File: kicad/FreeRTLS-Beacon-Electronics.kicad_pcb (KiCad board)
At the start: 2 copper layers, 27.1 x 52.5 mm, 37 parts, among them J1 USB_B_Micro, J2 STM Prog, U1 STM32F072CBTx, U2 AZ1117IH-3.3TRG1, U3 DWM1001

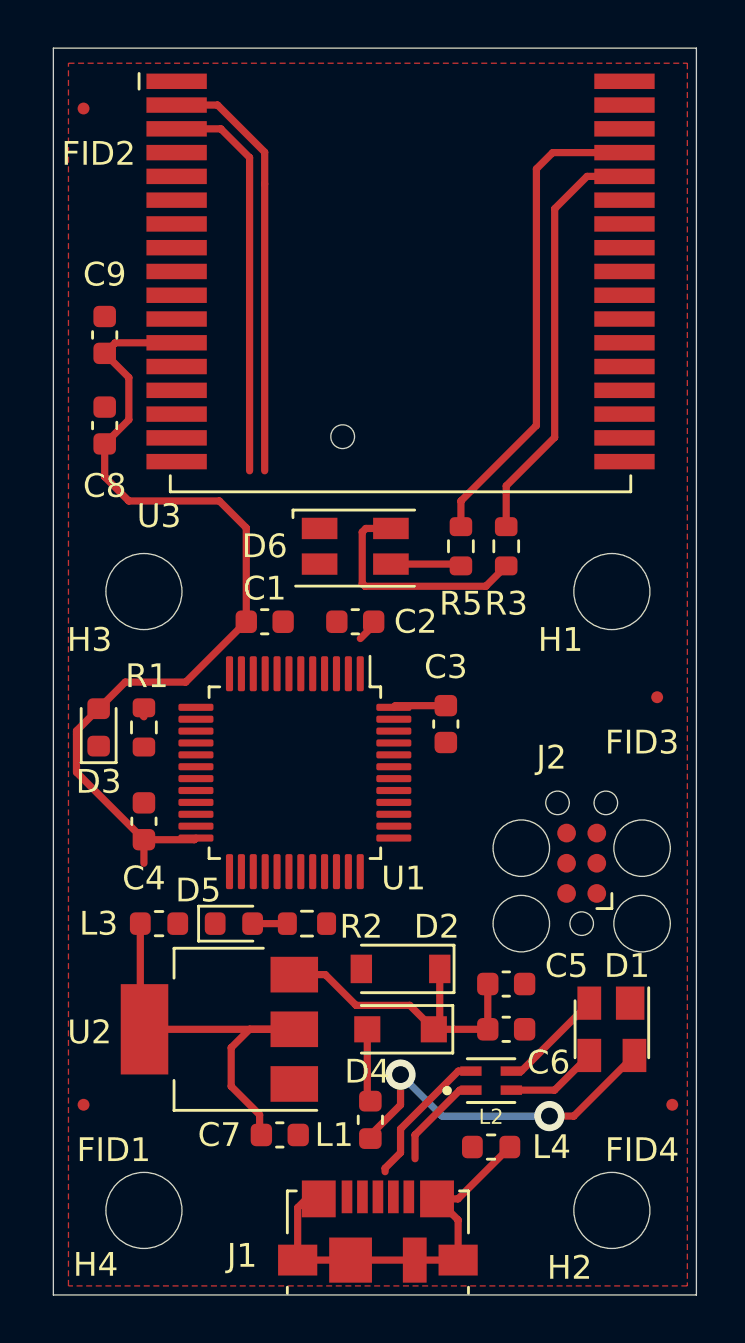
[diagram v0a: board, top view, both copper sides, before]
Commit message: Finish routing
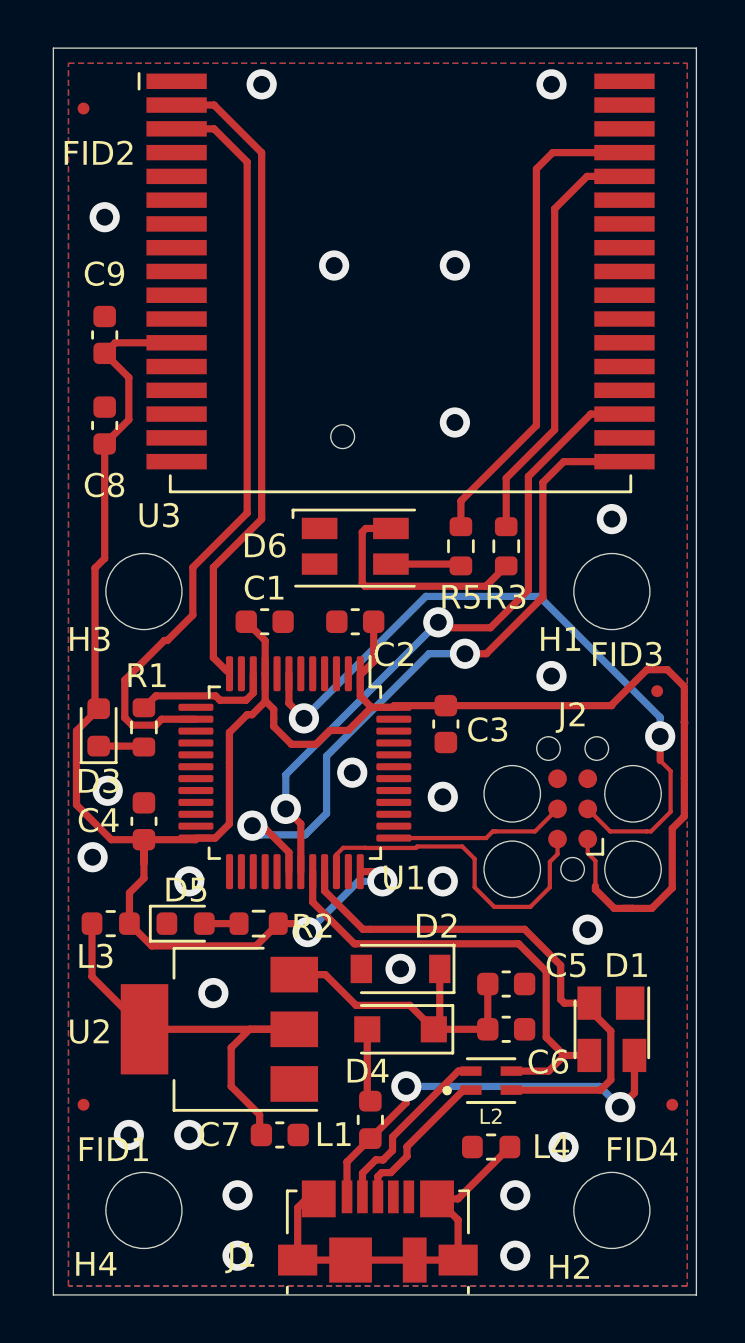
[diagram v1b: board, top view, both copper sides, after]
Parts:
- removed REF**: OSHW-Logo_5.7x6mm_SilkScreen, Symbol:OSHW-Logo_5.7x6mm_SilkScreen
- moved J2 2.32 mm to (135.5, 67.6)
- moved D5 2.03 mm to (119.2, 72.4)
- moved L3 2.03 mm to (116.1, 72.4)
- moved R2 2.03 mm to (122.3, 72.4)
- moved FID3 0.25 mm to (139.1, 62.6)
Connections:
- D1 pad 2: /MCU_D- -> /MCU_D+
- D1 pad 3: /MCU_D+ -> /MCU_D-
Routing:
- net +3V3: track 41.2 -> 98.7 mm, vias 0 -> 2
- net /STM_RESET: track 0.00 -> 30.1 mm, vias 0 -> 2
- net /TXD: track 0.00 -> 29.4 mm, vias 0 -> 2
- net /RXD: track 0.00 -> 27.9 mm, vias 0 -> 2
- net /MCU_D+: track 3.88 -> 22.7 mm
- net /SWDIO: track 16.7 -> 32.4 mm
- net /MCU_D-: track 4.46 -> 19.7 mm
- net Net-(J2-Pad2): track 0.00 -> 14.1 mm
- net /SWCLK: track 17.9 -> 27.3 mm
- net Net-(J2-Pad4): track 0.00 -> 7.39 mm
- net Net-(R1-Pad1): track 0.05 -> 5.82 mm
- net VBUS: track 14.8 -> 17.5 mm
- net Net-(J1-Pad3): track 4.13 -> 6.52 mm
- net Net-(D3-Pad1): track 0.00 -> 1.92 mm
- net Net-(J1-Pad2): track 6.04 -> 7.67 mm
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- added copper zone on B.Cu, net GND
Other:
- net class 10 added: clearance 0.254, trace_width 0.3048, via_dia 1.27, via_drill 0.7112
- net class 8/8 added: clearance 0.1778, trace_width 0.1778, via_dia 1.27, via_drill 0.7112
- net class Clear 7 added: clearance 0.1778, trace_width 0.3048, via_dia 1.27, via_drill 0.7112
- net class GND added: clearance 0.1778, trace_width 0.1778, via_dia 1.27, via_drill 0.7112
- rule trace_min: 0.3048 -> 0.1524

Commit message: Add PCBWay PCB Specification
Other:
- board text added: "PCBWay PCB Specification —————————————————— - Board type: Single pieces - Different Design in Panel: 1 - Size (single): 27.05 mm x 52.45 mm - Layers: 2 Layers - Material: FR-4 - FR4-TG: TG 130-140 - Thickness: 1.6 - Min Track/Spacing: 8/8 mil - Min Hole Size: 0.3 mm - Solder Mask: Purple (Prototype) - Black (Pre-Release) - Green (Release) - Silkscreen: White - Gold fingers: No - Surface Finish: H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"
